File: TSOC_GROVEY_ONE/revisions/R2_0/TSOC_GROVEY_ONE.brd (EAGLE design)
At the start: 44.5 x 30.5 mm, 53 parts, among them J3 NO, J4 6p-2.54, U1 MIC5219 3.3V, U2 ATMEGA328, X1 16MHZ

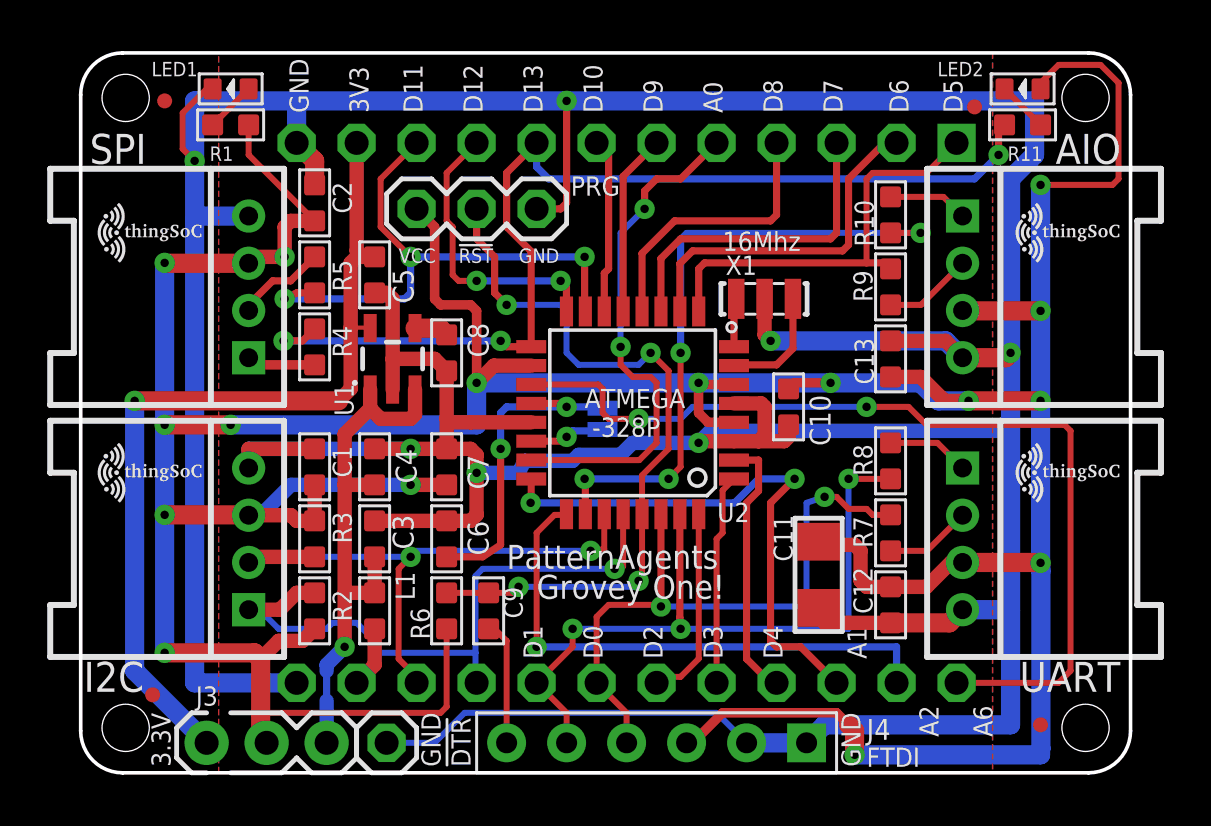
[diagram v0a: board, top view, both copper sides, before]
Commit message: update documetation
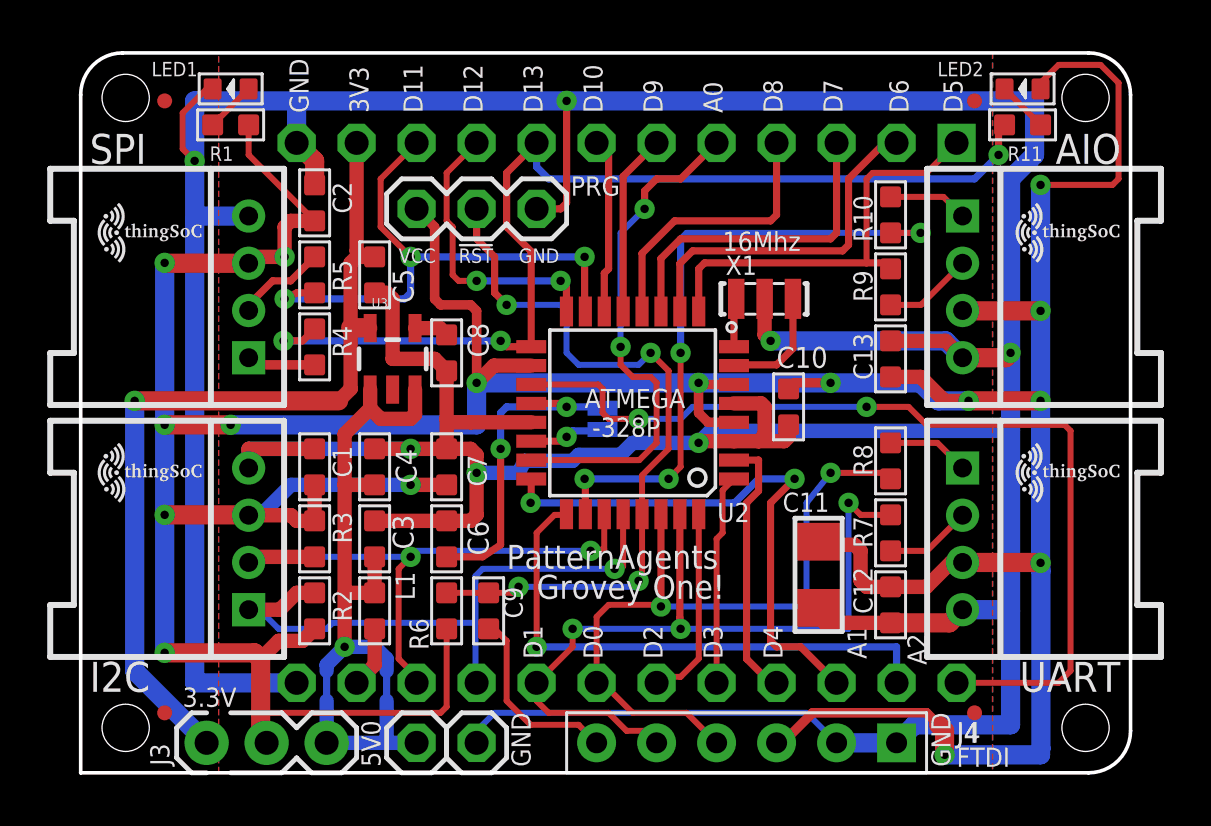
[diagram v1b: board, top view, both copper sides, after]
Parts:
- removed U1: MIC5219 3.3V, TSOC-ESP8266-BASE:SOT23-5
- added 5V0: (no value), PatternAgents-ProtoPads:1X01
- added U3: AP2112K-3.3V, SparkFun-PowerIC:SOT23-5
- moved GND 3.81 mm to (16.8, 1.27)
- moved J4 3.81 mm to (28.2, 1.27)
- moved FID4 2.84 mm to (37.8, 2.54)
- moved FID1 0.92 mm to (3.56, 2.54)
- moved FID3 0.25 mm to (37.8, 28.4)
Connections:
- net 3V3: now also U3.5; no longer U1.5
- net 5V0: now also 5V0.1, U3.1, U3.3; no longer U1.1, U1.3
- net BYPASS1: now also U3.4; no longer U1.4
- net D0: now also R8.1; no longer R7.1
- net D0E: now also R8.2, UART.1; no longer R7.2, UART.2
- net D1: now also R7.1; no longer R8.1
- net D1E: now also R7.2, UART.2; no longer R8.2, UART.1
- net GND: now also U3.2; no longer U1.2
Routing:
- net 5V0: track 23.0 -> 32.4 mm
- net GND: track 230.3 -> 225.5 mm
- net VCC: track 198.0 -> 194.2 mm
- net D0: track 27.2 -> 30.6 mm
- net !JRST: track 5.29 -> 8.06 mm
- net D1: track 30.6 -> 33.4 mm
- net A5: track 27.2 -> 26.3 mm
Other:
- outline, holes or cut-outs redrawn
